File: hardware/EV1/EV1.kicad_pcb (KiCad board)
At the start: 2 copper layers, 37 parts, among them J1 Conn_01x04_Male, J2 Conn_01x04_Male, J3 Conn_01x09_Male, J4 Conn_01x07_Male, J5 Conn_01x08_Male, J6 Conn_01x04_Male, J7 Conn_01x06_Male, P1 USB_C_Plug, SW1 SW_SPDT, SW2 SW_Push, U1 STM32F405RGTx, U2 AMS1117-3.3, Y1 25mhz

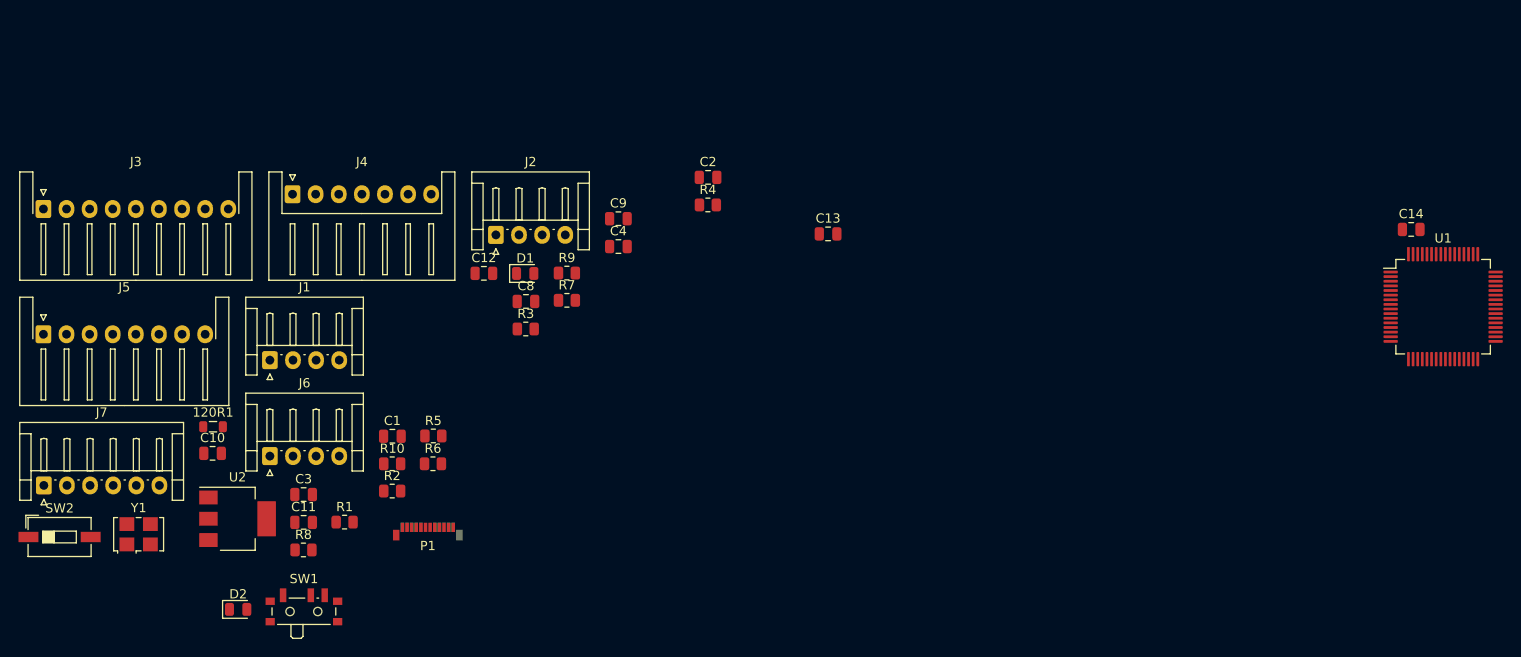
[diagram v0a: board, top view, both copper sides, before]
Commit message: Finished Version of EV1
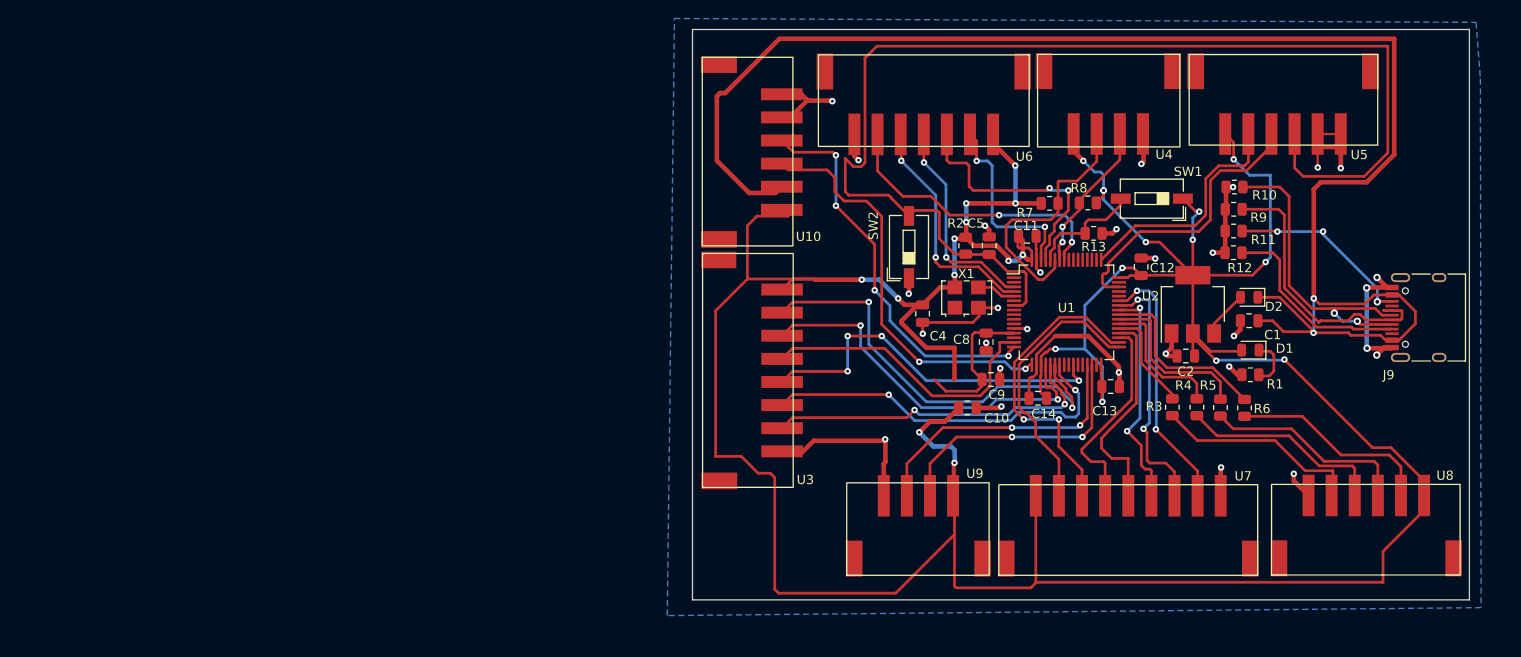
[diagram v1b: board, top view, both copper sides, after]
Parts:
- removed 120R1: FerriteBead, Inductor_SMD:L_0805_2012Metric
- removed C3: 10p, Capacitor_SMD:C_0805_2012Metric
- removed J1, J2, J6: Conn_01x04_Male, Connector_JST:JST_EH_S4B-EH_1x04_P2.50mm_Horizontal
- removed J3: Conn_01x09_Male, Connector_JST:JST_XH_S9B-XH-A-1_1x09_P2.50mm_Horizontal
- removed J4: Conn_01x07_Male, Connector_JST:JST_XH_S7B-XH-A_1x07_P2.50mm_Horizontal
- removed J5: Conn_01x08_Male, Connector_JST:JST_XH_S8B-XH-A-1_1x08_P2.50mm_Horizontal
- removed J7: Conn_01x06_Male, Connector_JST:JST_EH_S6B-EH_1x06_P2.50mm_Horizontal
- removed P1: USB_C_Plug, Connector_USB:USB_C_Plug_Molex_105444
- removed Y1: 25mhz, Oscillator:Oscillator_SMD_SeikoEpson_SG8002LB-4Pin_5.0x3.2mm
- added C5: 100n, Capacitor_SMD:C_0805_2012Metric, F.Cu at (145.9, 84.6)
- added J9: USB_C_Receptacle, Connector_USB:USB_C_Receptacle_HRO_TYPE-C-31-M-12, F.Cu at (193.5, 92.4)
- added R11: 5k1, Resistor_SMD:R_0805_2012Metric, F.Cu at (172.3, 83.0)
- added R12: 5k1, Resistor_SMD:R_0805_2012Metric, F.Cu at (172.3, 85.3)
- added R13: 4k7, Resistor_SMD:R_0805_2012Metric, F.Cu at (157.2, 83.3)
- added U10: 1x6_connector, 1x4 pin download:1x6_connector, F.Cu at (123.4, 68.2)
- added U3: 1x8_connector, 1x4 pin download:1X8_CONNECTOR, F.Cu at (123.5, 89.3)
- added U4: 1x4_connector, 1x4 pin download:1x4_connector, F.Cu at (162.5, 72.5)
- added U5: 1x6_connector, 1x4 pin download:1x6_connector, F.Cu at (183.9, 72.5)
- added U6: 1x7_connector, 1x4 pin download:1x7_connector, F.Cu at (146.3, 72.5)
- added U7: 1x9_connector, 1x4 pin download:1x9_connector, F.Cu at (150.9, 111.6)
- added U8: 1x6_connector, 1x4 pin download:1x6_connector, F.Cu at (180.4, 111.6)
- added U9: 1x4_connector, 1x4 pin download:1x4_connector, F.Cu at (134.5, 111.6)
- added X1: SG-5032CAN, Oscillator:Oscillator_SMD_SeikoEpson_SG8002LB-4Pin_5.0x3.2mm, F.Cu at (143.4, 90.2)
- C4: value 10p -> 100n
- R1: value 130 -> 150
- R2: value 10k -> 4k7
- SW1: value SW_SPDT -> SW_Push; footprint Button_Switch_SMD:SW_SPDT_PCM12 -> Button_Switch_SMD:SW_DIP_SPSTx01_Slide_6.7x4.1mm_W6.73mm_P2.54mm_LowProfile_JPin
- moved D2 114.5 mm to (174.0, 90.2), turned to 180 degrees
- moved U2 105.9 mm to (167.9, 90.9), turned to 90 degrees
- moved SW1 101.9 mm to (163.5, 79.5), turned to 180 degrees
- moved R1 99.3 mm to (174.1, 98.6)
- moved SW2 97.1 mm to (137.2, 84.7), turned to 90 degrees
- moved R10 95.9 mm to (172.4, 78.2)
- moved C1 93.5 mm to (174.0, 92.7), turned to 180 degrees
- moved R8 92.8 mm to (156.5, 80.0), turned to 180 degrees
- moved R6 88.0 mm to (173.5, 102.1), turned to 90 degrees
- moved R5 85.2 mm to (170.9, 102.1), turned to 90 degrees
- moved C11 84.2 mm to (150.0, 83.6)
- moved C10 81.8 mm to (143.5, 102.1)
- moved D1 78.9 mm to (174.1, 95.9), turned to 180 degrees
- moved R9 72.5 mm to (172.3, 80.7)
- moved C12 71.1 mm to (162.3, 86.9), turned to 90 degrees
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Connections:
- C4 pad 1: /HSE_OUT -> +3.3V
- D2 pad 2: VBUS -> Net-(D2-Pad2)
- R2 pad 1: /SW_BOOT0 -> /RESET
- R2 pad 2: /BOOT0 -> +3.3V
- SW1 pad 1: GND -> +3.3V
- SW1 pad 2: /SW_BOOT0 -> /BOOT0
- SW2 pad 1: Net-(SW2-Pad1) -> GND
- SW2 pad 2: +3.3V -> /RESET
- U1 pad 46: unconnected-(U1-Pad46) -> /SWD_DIO
- U1 pad 49: unconnected-(U1-Pad49) -> /SWD_CLK
- U1 pad 6: /HSE_OUT -> unconnected-(U1-Pad6)
- U1 pad 7: Net-(SW2-Pad1) -> /RESET
- U2 pad 3: VBUS -> Net-(D2-Pad2)
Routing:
- net +3.3V: track 0.00 -> 403.5 mm, vias 0 -> 25
- net VBUS: track 0.00 -> 169.2 mm, vias 0 -> 2
- net /RESET: track 0.00 -> 129.9 mm
- net GND: track 0.00 -> 129.8 mm, vias 0 -> 29
- net /RST_PA6: track 0.00 -> 47.4 mm, vias 0 -> 2
- net /USART2_RX: track 0.00 -> 44.2 mm, vias 0 -> 2
- net /USART2_TX: track 0.00 -> 42.5 mm, vias 0 -> 4
- net /MOSI_SPI: track 0.00 -> 40.7 mm, vias 0 -> 2
- net /BL_PA4: track 0.00 -> 40.4 mm, vias 0 -> 2
- net /DC_PB0: track 0.00 -> 40.4 mm, vias 0 -> 4
- net /SCK_SPI: track 0.00 -> 38.2 mm, vias 0 -> 2
- net Net-(J9-PadA7): track 0.00 -> 34.9 mm, vias 0 -> 2
- net /BB_ROW_3: track 0.00 -> 34.2 mm, vias 0 -> 2
- net /CS_PA1: track 0.00 -> 32.2 mm
- net /BB_COLS_6: track 0.00 -> 31.7 mm, vias 0 -> 2
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- added copper zone on B.Cu, net GND
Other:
- board outline added: 84 x 61.7 mm
